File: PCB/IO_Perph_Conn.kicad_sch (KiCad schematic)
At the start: 17 parts, among them U4 STM32MP157FABx, Y1 NX2012SA-32.768K

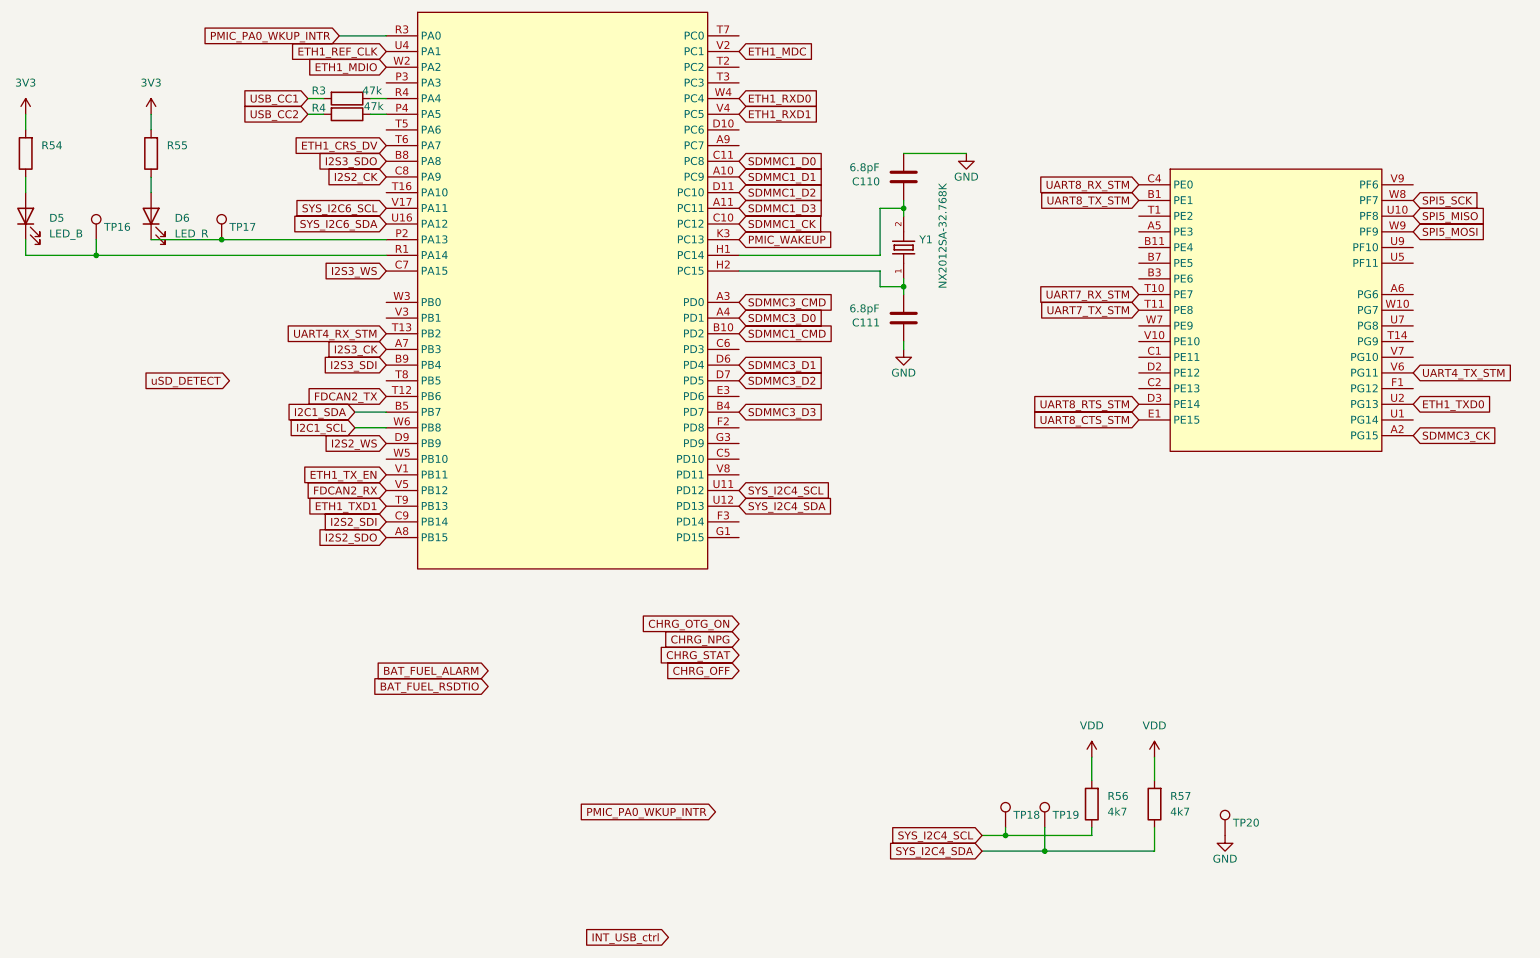
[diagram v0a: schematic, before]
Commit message: update
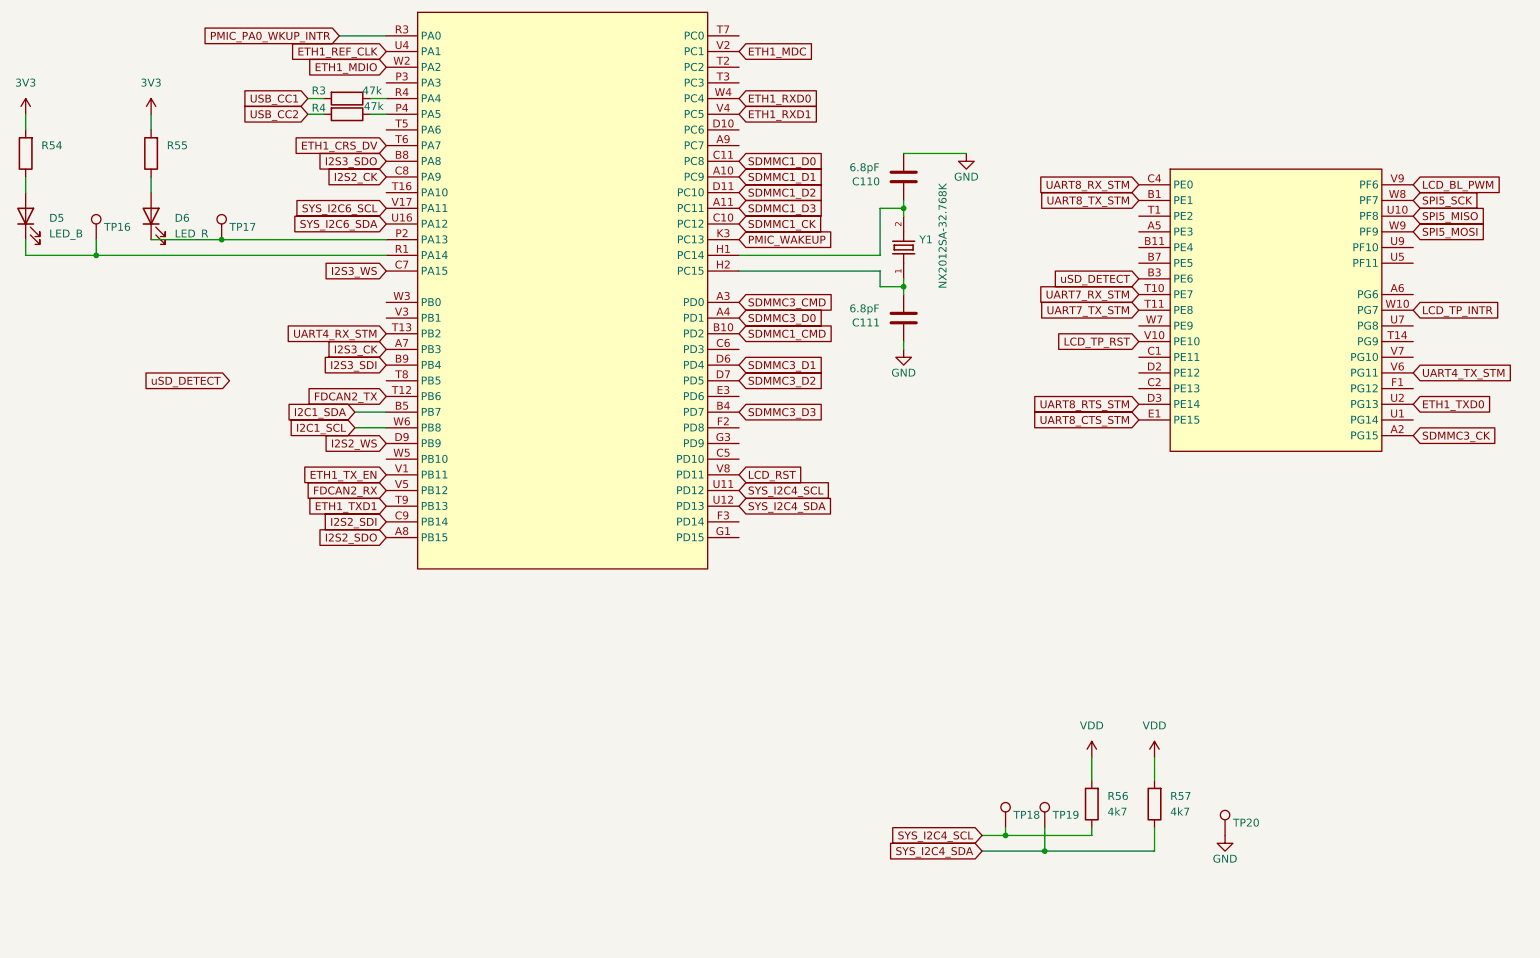
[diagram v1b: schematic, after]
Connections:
- net uSD_DETECT: now also U4.B3 (PE6)
- net LCD_TP_RST: now reaches U4.V10 (PE10)
- net LCD_BL_PWM: now reaches U4.V9 (PF6)
- net LCD_TP_INTR: now reaches U4.W10 (PG7)
- net LCD_RST: now reaches U4.V8 (PD11)
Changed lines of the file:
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@@
 				)
 			)
-			(table_cell ""
+			(table_cell "LCD_BL_PWM"
 				(exclude_from_sim no)
 				(at 330.2 205.74 0)
@@
 				)
 			)
-			(table_cell ""
+			(table_cell "PF6"
 				(exclude_from_sim no)
 				(at 354.33 205.74 0)
@@
 				)
 			)
-			(table_cell ""
+			(table_cell "V9"
 				(exclude_from_sim no)
 				(at 378.46 205.74 0)
@@
 		)
 	)
-	(global_label "CHRG_STAT"
-		(shape input)
-		(at 162.56 151.13 180)
-		(fields_autoplaced yes)
-		(effects
-			(font
-				(size 1.27 1.27)
-			)
-			(justify right)
-		)
-		(property "Intersheetrefs" "${INTERSHEET_REFS}"
-			(at 149.2334 151.13 0)
-			(effects
-				(font
-					(size 1.27 1.27)
-				)
-				(justify right)
-				(hide yes)
-			)
-		)
-	)
 	(global_label "SDMMC1_D0"
 		(shape input)
@@
 		)
 	)
+	(global_label "LCD_BL_PWM"
+		(shape input)
+		(at 271.78 74.93 0)
+		(fields_autoplaced yes)
+		(effects
+			(font
+				(size 1.27 1.27)
+			)
+			(justify left)
+		)
+		(property "Intersheetrefs" "${INTERSHEET_REFS}"
+			(at 286.7394 74.93 0)
+			(effects
+				(font
+					(size 1.27 1.27)
+				)
+				(justify left)
+				(hide yes)
+			)
+		)
+	)
 	(global_label "SYS_I2C6_SDA"
 		(shape input)
@@
 		)
 	)
-	(global_label "CHRG_OTG_ON"
-		(shape input)
-		(at 162.56 146.05 180)
-		(fields_autoplaced yes)
-		(effects
-			(font
-				(size 1.27 1.27)
-			)
-			(justify right)
-		)
-		(property "Intersheetrefs" "${INTERSHEET_REFS}"
-			(at 146.27 146.05 0)
+	(global_label "uSD_DETECT"
+		(shape input)
+		(at 227.33 90.17 180)
+		(fields_autoplaced yes)
+		(effects
+			(font
+				(size 1.27 1.27)
+			)
+			(justify right)
+		)
+		(property "Intersheetrefs" "${INTERSHEET_REFS}"
+			(at 212.9755 90.17 0)
 			(effects
 				(font
@@
 		)
 	)
+	(global_label "LCD_TP_RST"
+		(shape input)
+		(at 227.33 100.33 180)
+		(fields_autoplaced yes)
+		(effects
+			(font
+				(size 1.27 1.27)
+			)
+			(justify right)
+		)
+		(property "Intersheetrefs" "${INTERSHEET_REFS}"
+			(at 213.1568 100.33 0)
+			(effects
+				(font
+					(size 1.27 1.27)
+				)
+				(justify right)
+				(hide yes)
+			)
+		)
+	)
 	(global_label "SDMMC3_D3"
 		(shape input)
@@
 		)
 	)
-	(global_label "INT_USB_ctrl"
-		(shape input)
-		(at 151.13 196.85 180)
-		(fields_autoplaced yes)
-		(effects
-			(font
-				(size 1.27 1.27)
-			)
-			(justify right)
-		)
-		(property "Intersheetrefs" "${INTERSHEET_REFS}"
-			(at 136.231 196.85 0)
-			(effects
-				(font
-					(size 1.27 1.27)
-				)
-				(justify right)
+	(global_label "LCD_RST"
+		(shape input)
+		(at 162.56 121.92 0)
+		(fields_autoplaced yes)
+		(effects
+			(font
+				(size 1.27 1.27)
+			)
+			(justify left)
+		)
+		(property "Intersheetrefs" "${INTERSHEET_REFS}"
+			(at 173.528 121.92 0)
+			(effects
+				(font
+					(size 1.27 1.27)
+				)
+				(justify left)
 				(hide yes)
 			)
@@
 		)
 	)
-	(global_label "CHRG_NPG"
-		(shape input)
-		(at 162.56 148.59 180)
-		(fields_autoplaced yes)
-		(effects
-			(font
-				(size 1.27 1.27)
-			)
-			(justify right)
-		)
-		(property "Intersheetrefs" "${INTERSHEET_REFS}"
-			(at 149.5962 148.59 0)
-			(effects
-				(font
-					(size 1.27 1.27)
-				)
-				(justify right)
+	(global_label "LCD_TP_INTR"
+		(shape input)
+		(at 271.78 95.25 0)
+		(fields_autoplaced yes)
+		(effects
+			(font
+				(size 1.27 1.27)
+			)
+			(justify left)
+		)
+		(property "Intersheetrefs" "${INTERSHEET_REFS}"
+			(at 286.679 95.25 0)
+			(effects
+				(font
+					(size 1.27 1.27)
+				)
+				(justify left)
 				(hide yes)
 			)
@@
 		)
 	)
-	(global_label "CHRG_OFF"
-		(shape input)
-		(at 162.56 153.67 180)
-		(fields_autoplaced yes)
-		(effects
-			(font
-				(size 1.27 1.27)
-			)
-			(justify right)
-		)
-		(property "Intersheetrefs" "${INTERSHEET_REFS}"
-			(at 149.959 153.67 0)
-			(effects
-				(font
-					(size 1.27 1.27)
-				)
-				(justify right)
-				(hide yes)
-			)
-		)
-	)
-	(global_label "BAT_FUEL_ALARM"
-		(shape input)
-		(at 121.92 153.67 180)
-		(fields_autoplaced yes)
-		(effects
-			(font
-				(size 1.27 1.27)
-			)
-			(justify right)
-		)
-		(property "Intersheetrefs" "${INTERSHEET_REFS}"
-			(at 103.1505 153.67 0)
-			(effects
-				(font
-					(size 1.27 1.27)
-				)
-				(justify right)
-				(hide yes)
-			)
-		)
-	)
 	(global_label "SDMMC1_D1"
 		(shape input)
@@
 		)
 	)
-	(global_label "PMIC_PA0_WKUP_INTR"
-		(shape input)
-		(at 158.75 176.53 180)
-		(fields_autoplaced yes)
-		(effects
-			(font
-				(size 1.27 1.27)
-			)
-			(justify right)
-		)
-		(property "Intersheetrefs" "${INTERSHEET_REFS}"
-			(at 135.2029 176.53 0)
-			(effects
-				(font
-					(size 1.27 1.27)
-				)
-				(justify right)
-				(hide yes)
-			)
-		)
-	)
 	(global_label "SPI5_MOSI"
 		(shape input)
@@
 				(hide yes)
 			)
-		)
-	)
-	(global_label "BAT_FUEL_RSDTIO"
-		(shape input)
-		(at 121.92 156.21 180)
-		(fields_autoplaced yes)
-		(effects
-			(font
-				(size 1.27 1.27)
-			)
-			(justify right)
-		)
-		(property "Intersheetrefs" "${INTERSHEET_REFS}"
-			(at 102.4248 156.21 0)
-			(effects
-				(font
-					(size 1.27 1.27)
-				)
-				(justify right)
-				(hide yes)
-			)
